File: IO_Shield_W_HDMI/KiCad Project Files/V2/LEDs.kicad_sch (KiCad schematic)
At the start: 70 parts, among them Q1 FDN340P, Q2 FDN340P, Q3 FDN340P, Q4 FDN340P, SW1 SW_DIP_x08, SW2 SW_DIP_x08

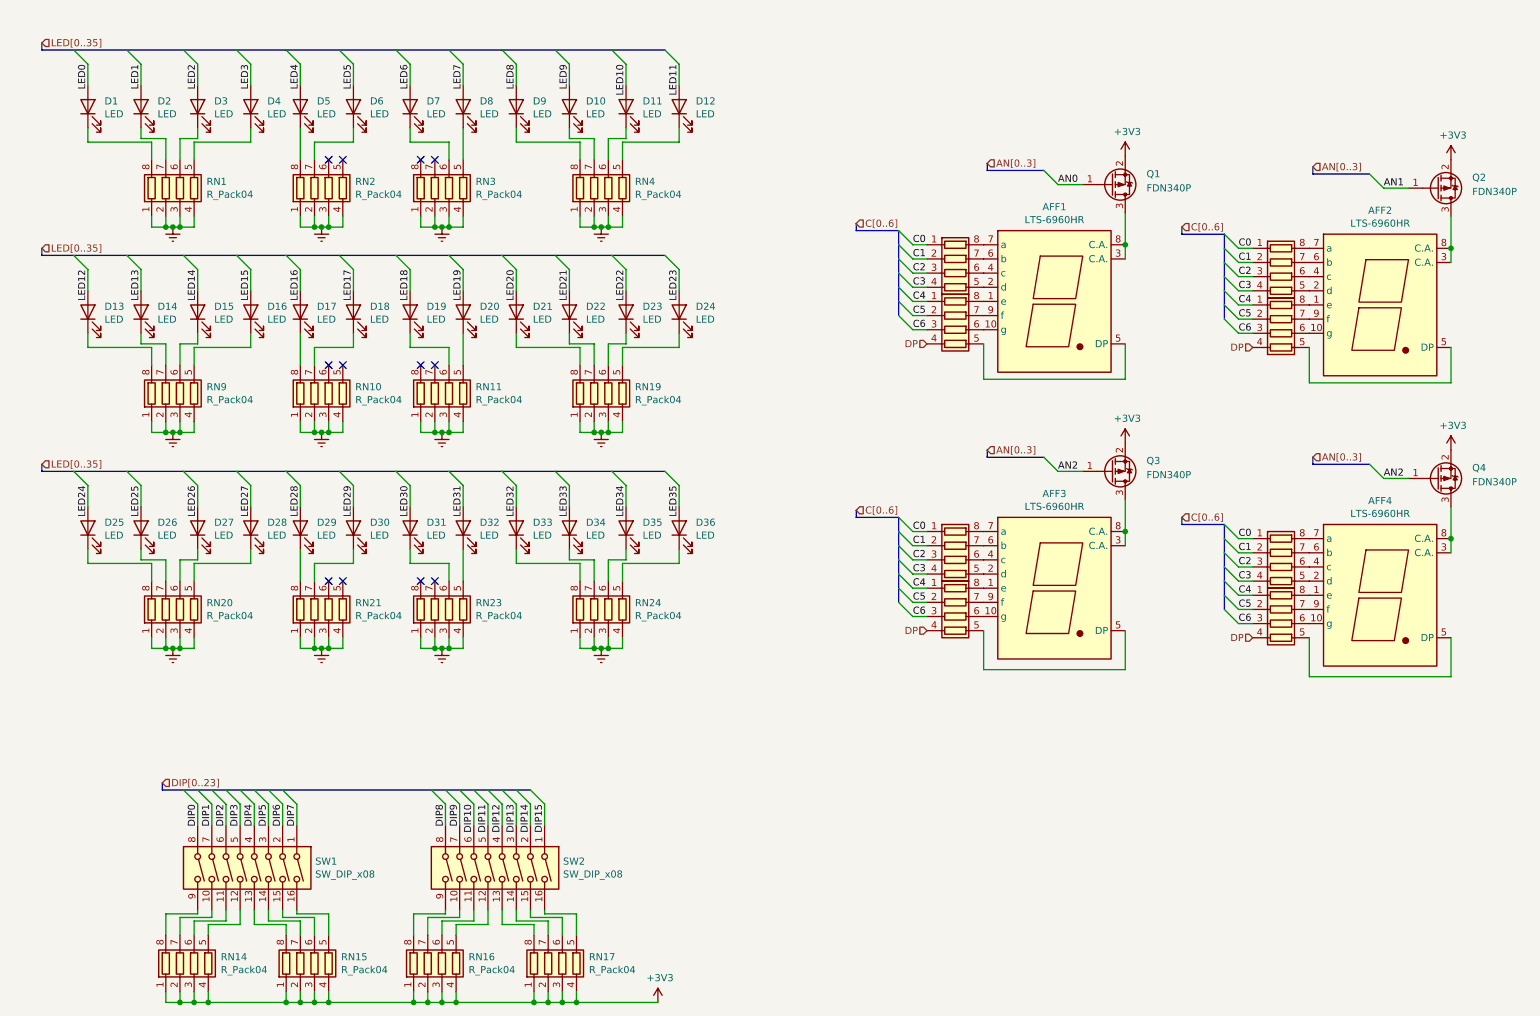
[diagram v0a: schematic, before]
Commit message: working on placement
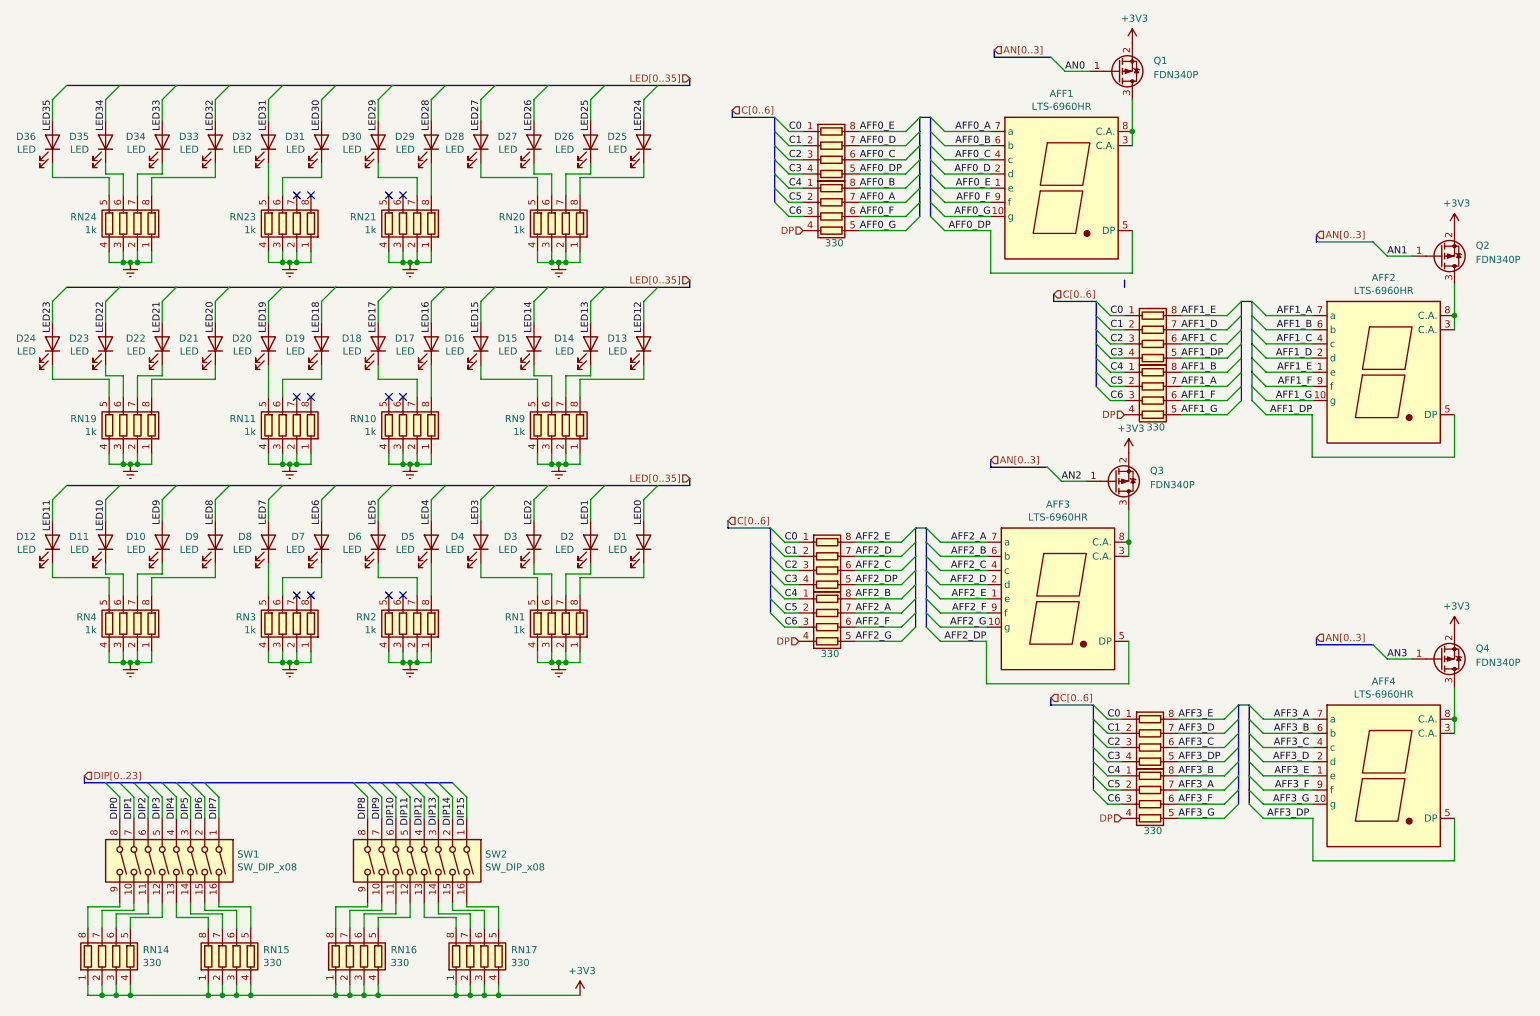
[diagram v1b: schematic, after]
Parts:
- RN1, RN10, RN11, RN19, RN2, RN20, RN21, RN23, RN24, RN3, RN4, RN9: value R_Pack04 -> 1k
- RN13, RN14, RN15, RN16, RN17, RN22, RN7, RN8: value R_Pack04 -> 330
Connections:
- net AN2: no longer Q4.1 (G)
- net AFF0_B: now reaches RN7.8 (R1.2)
- net AFF0_B: now also AFF1.6 (b); no longer AFF1.1 (e)
- net AFF0_F: now reaches RN7.6 (R3.2)
- net AFF0_F: now also AFF1.9 (f); no longer AFF1.10 (g)
- net AFF0_D: now reaches AFF1.2 (d)
- net AFF0_D: now also RN5.7 (R2.2); no longer RN5.5 (R4.2)
- net AFF0_C: now reaches AFF1.4 (c), RN5.6 (R3.2)
- net AFF0_DP: now reaches AFF1.5 (DP)
- net AFF0_DP: now also RN5.5 (R4.2); no longer RN7.5 (R4.2)
- net AFF0_A: now reaches AFF1.7 (a)
- net AFF0_A: now also RN7.7 (R2.2); no longer RN5.8 (R1.2)
- net AFF1_B: now reaches RN8.8 (R1.2)
- net AFF1_B: now also AFF2.6 (b); no longer AFF2.1 (e)
- net AFF1_F: now reaches RN8.6 (R3.2)
- net AFF1_F: now also AFF2.9 (f); no longer AFF2.10 (g)
- net AFF1_D: now reaches AFF2.2 (d)
- net AFF1_D: now also RN6.7 (R2.2); no longer RN6.5 (R4.2)
- net AFF1_C: now reaches AFF2.4 (c), RN6.6 (R3.2)
- net AFF1_DP: now reaches AFF2.5 (DP)
- net AFF1_DP: now also RN6.5 (R4.2); no longer RN8.5 (R4.2)
- net AFF1_A: now reaches AFF2.7 (a)
- net AFF1_A: now also RN8.7 (R2.2); no longer RN6.8 (R1.2)
- net AFF2_B: now reaches RN13.8 (R1.2)
- net AFF2_B: now also AFF3.6 (b); no longer AFF3.1 (e)
- net AFF2_F: now reaches RN13.6 (R3.2)
- net AFF2_F: now also AFF3.9 (f); no longer AFF3.10 (g)
- net AFF2_D: now reaches AFF3.2 (d)
- net AFF2_D: now also RN12.7 (R2.2); no longer RN12.5 (R4.2)
- net AFF2_C: now reaches AFF3.4 (c), RN12.6 (R3.2)
- net AFF2_DP: now reaches AFF3.5 (DP)
- net AFF2_DP: now also RN12.5 (R4.2); no longer RN13.5 (R4.2)
- net AFF2_A: now reaches AFF3.7 (a)
- net AFF2_A: now also RN13.7 (R2.2); no longer RN12.8 (R1.2)
- net AFF3_DP: now reaches AFF4.5 (DP)
- net AFF3_DP: now also RN18.5 (R4.2); no longer RN22.5 (R4.2)
- net AFF3_F: now reaches RN22.6 (R3.2)
- net AFF3_F: now also AFF4.9 (f); no longer AFF4.10 (g)
- net AFF3_A: now reaches RN22.7 (R2.2)
- net AFF3_A: now also AFF4.7 (a); no longer AFF4.9 (f)
- net AFF3_B: now reaches RN22.8 (R1.2)
- net AFF3_B: now also AFF4.6 (b); no longer AFF4.1 (e)
- net AFF3_D: now reaches AFF4.2 (d)
- net AFF3_D: now also RN18.7 (R2.2); no longer RN18.5 (R4.2)
- net AFF3_C: now reaches AFF4.4 (c), RN18.6 (R3.2)
- net AFF3_E: now reaches RN18.8 (R1.2)
- net AFF3_E: now also AFF4.1 (e); no longer AFF4.7 (a)
- new net AFF0_E: AFF1.1 (e), RN5.8 (R1.2)
- new net AFF0_G: AFF1.10 (g), RN7.5 (R4.2)
- new net AFF1_E: AFF2.1 (e), RN6.8 (R1.2)
- new net AFF1_G: AFF2.10 (g), RN8.5 (R4.2)
- new net AFF2_E: AFF3.1 (e), RN12.8 (R1.2)
- new net AFF2_G: AFF3.10 (g), RN13.5 (R4.2)
- new net AFF3_G: AFF4.10 (g), RN22.5 (R4.2)
- new net AN3: Q4.1 (G)
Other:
- moved on the sheet: AFF1, AFF2, AFF3, AFF4, D1, D10, D11, D12, D13, D14, D15, D16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
